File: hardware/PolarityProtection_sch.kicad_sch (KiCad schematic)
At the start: 19 parts, among them IC1 LM74502HDDFR, Q1 NVMFWS1D7N04XMT1G, Q4 NVMFWS1D7N04XMT1G

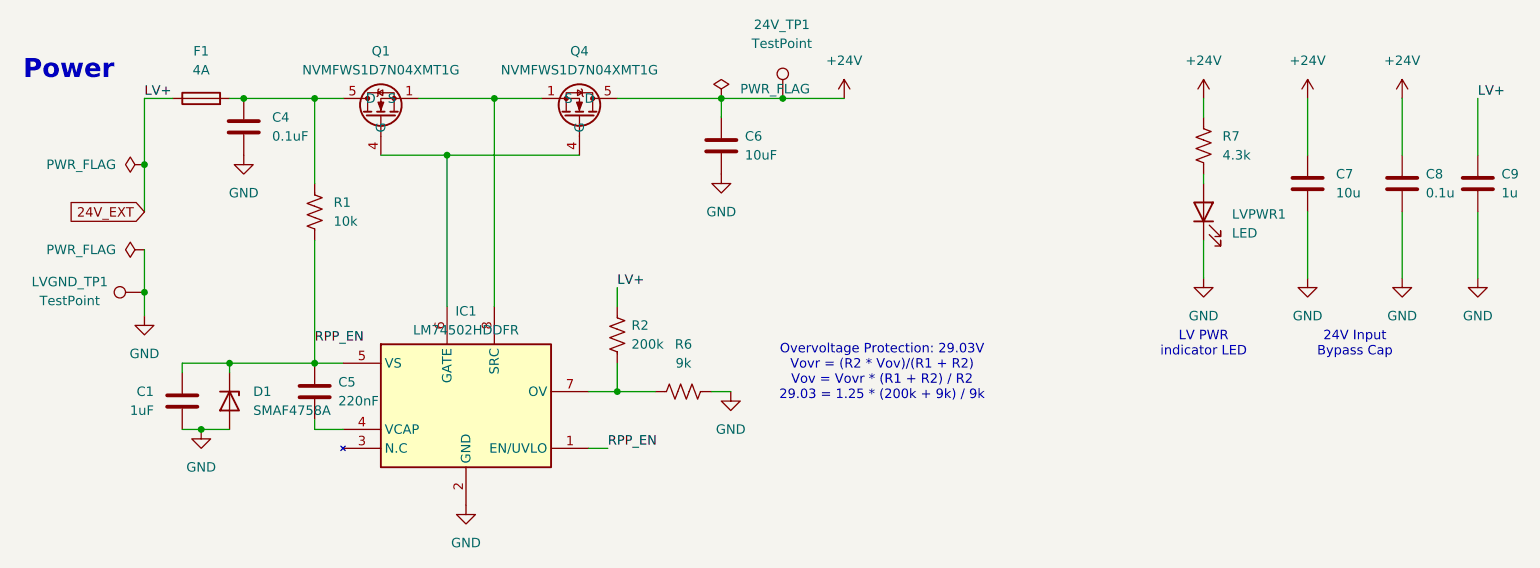
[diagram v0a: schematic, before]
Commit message: Current Layout
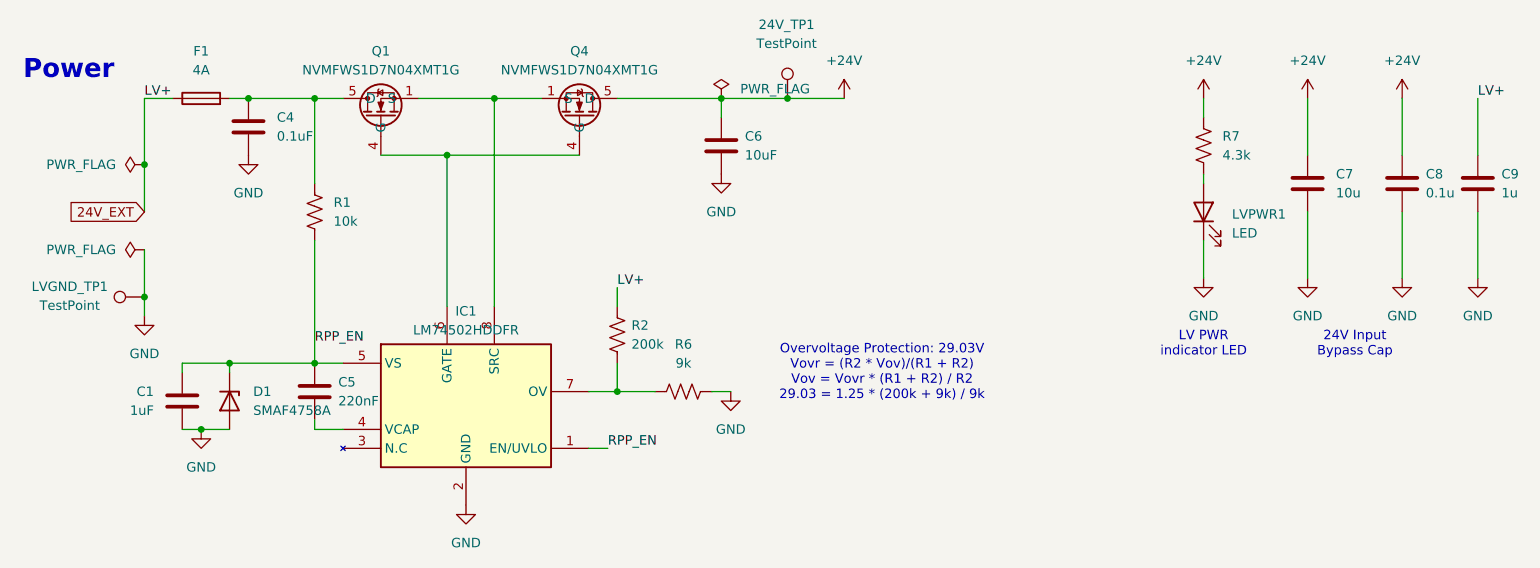
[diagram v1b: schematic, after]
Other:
- moved on the sheet: 24V_TP1, C4, LVGND_TP1
